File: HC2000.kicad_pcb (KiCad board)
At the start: 2 copper layers, 478 x 183 mm, 259 parts, among them J1 VIDEO, J10 SDS-60J, J2 JOYSTICK, J3 >VALUE, J4 ., J5 RS232 + RETEA, J6 ., J7 FDD-CON, J8 FDD-CON, J9 ., Q1 17,734, Q2 8MHz, SW1 >VALUE, T1 BD139, T2 2N2369/2N2368, T3 2N2369/BC108A, T4 BC177, T5 BC177

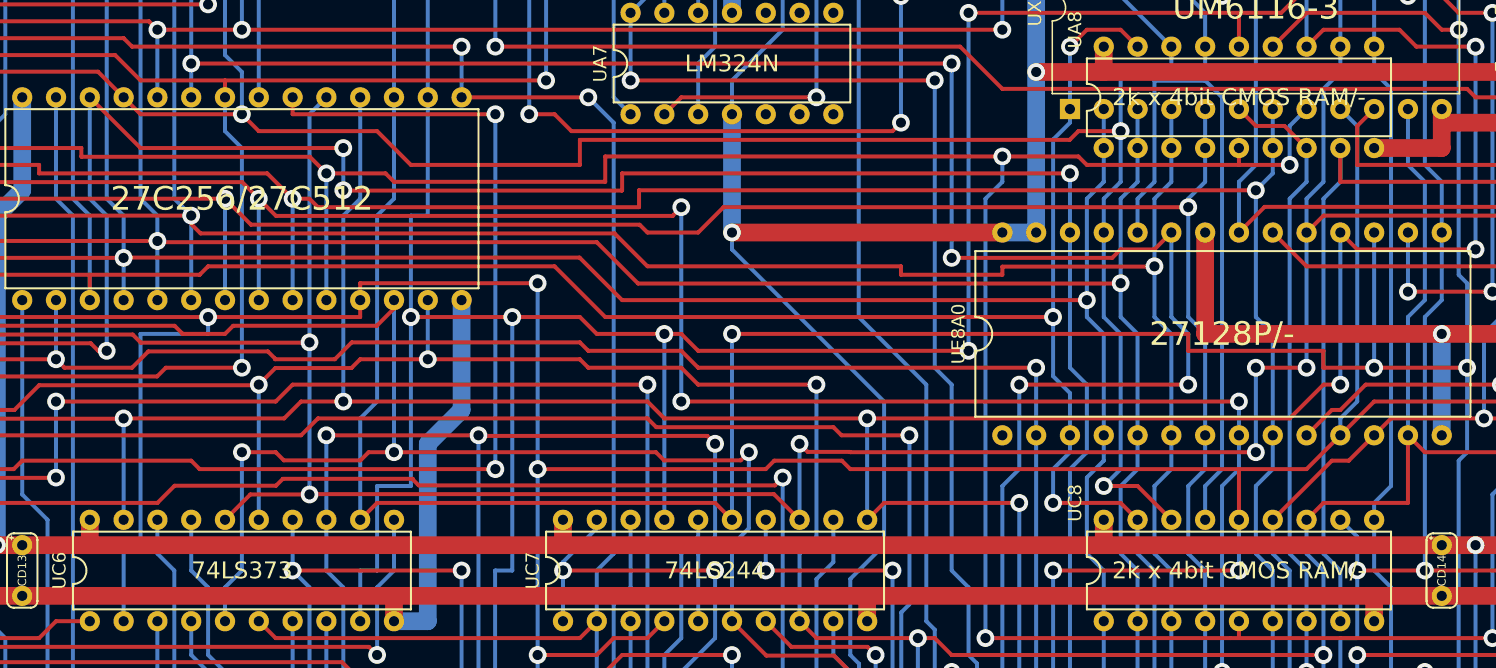
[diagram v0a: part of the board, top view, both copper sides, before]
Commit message: Revision-E
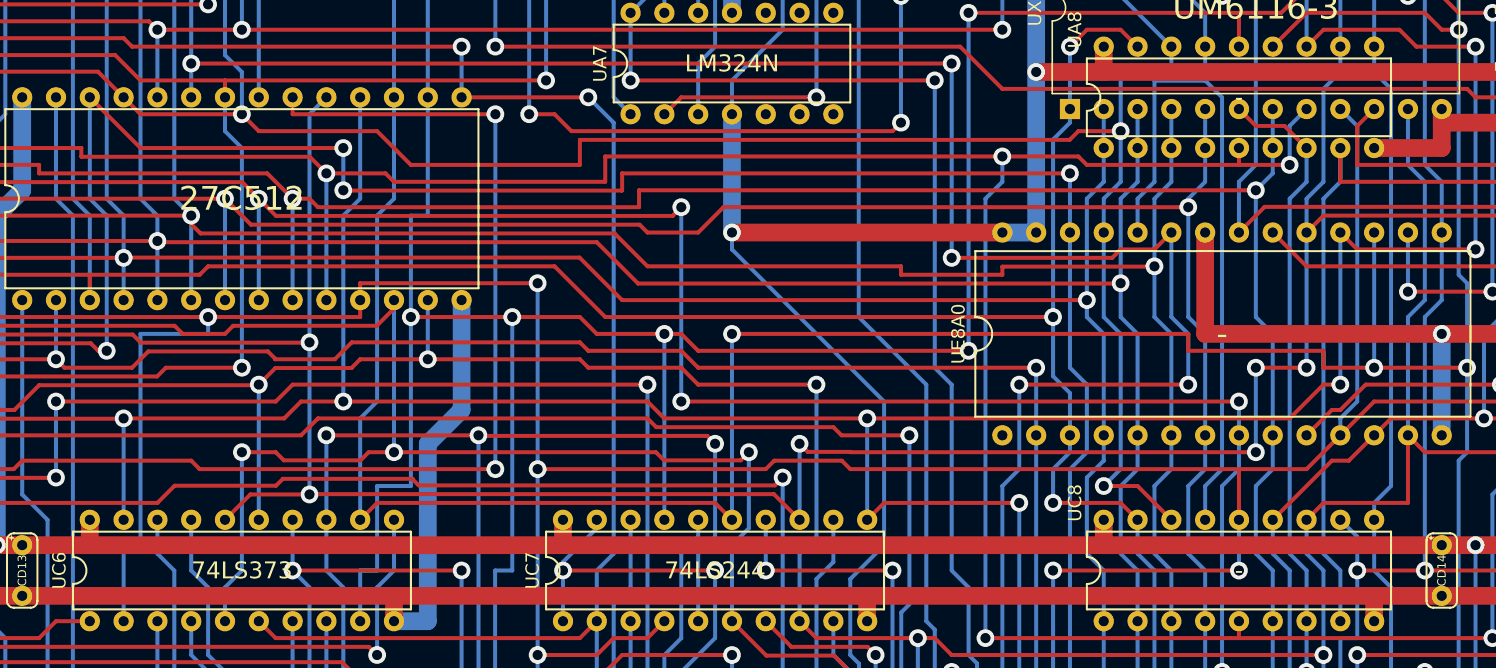
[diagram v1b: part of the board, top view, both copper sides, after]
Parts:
- C14: value 100p/180p -> 180p
- C4: value 3,3uF/4,7uF -> 4,7uF
- C7: value 10p/15p -> 15p
- C8: value 220p/- -> -
- J3: value >VALUE -> MAB5SH
- R21: value 10k/470k -> 470k
- R22: value 8k2/6k -> 6k
- R26, R42, R45: value 330/- -> -
- R28, R40, R41, R56: value 220/1k -> 1k
- R30, R48: value 75/69 -> 69
- R31: value 240/270 -> 270
- R5, R60: value 330/300 -> 300
- R6: value 2M2/2M -> 2M
- R66: value 1k8/1k6 -> 1k6
- R68: value 5k6/5k1 -> 5k1
- SW1: value >VALUE -> RESET_SW
- T2: value 2N2369/2N2368 -> 2N2368
- T3: value 2N2369/BC108A -> BC108A
- UA8, UC8: value 2k x 4bit CMOS RAM/- -> -
- UB6: value 27C256/27C512 -> 27C512
- UE8A0: value 27128P/- -> -
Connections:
- JX2 pad 2: Net-(JX2-B) -> Net-(JX1-A)
- JX3 pad 2: Net-(JX3-B) -> Net-(JX3-A)
- JX4 pad 1: Net-(JX4-A) -> ROMFDD
- UA8 pad 8: Net-(JX3-B) -> Net-(JX3-A)
- UB10 pad 14: Net-(JX3-B) -> Net-(JX3-A)
- UC8 pad 8: Net-(JX3-B) -> Net-(JX3-A)
- UD11 pad 12: Net-(JX2-B) -> Net-(JX1-A)
- UF10 pad 6: Net-(JX4-A) -> ROMFDD
- UX1 pad 18: Net-(JX3-B) -> Net-(JX3-A)
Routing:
- net Net-(JX3-B): track 225.4 -> 0.00 mm, vias 8 -> 0
- net Net-(JX3-A): track 7.16 -> 232.5 mm, vias 0 -> 8
- net Net-(JX1-A): track 225.9 -> 230.6 mm
- net Net-(JX2-B): track 4.68 -> 0.00 mm
- net ROMFDD: track 366.2 -> 370.8 mm
- net Net-(JX4-A): track 4.55 -> 0.00 mm
